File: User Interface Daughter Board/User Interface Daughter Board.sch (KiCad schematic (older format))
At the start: 27 parts, among them J1 Mother Board Conn, J2 Jack-DC, SW1 SW_Push_DPDT_2-5_3-4_1-4, SW2 SW_Push_Dual_1-3_2-4, SW3 SW_Push_Dual_1-3_2-4, SW4 SW_Push_Dual_1-3_2-4

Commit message: Update JST connectors
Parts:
- J1: footprint Naquadah_Generator:Daughter_Board_Vert_6_Pin_JST_Conn -> Connector_JST:JST_SH_BM06B-SRSS-TB_1x06-1MP_P1.00mm_Vertical
- WA1: footprint Naquadah_Generator:Wire_Assembly_Four -> Mechanical_LE:Wire_Assembly; symbol Naquadah_Generator:WireAssembly -> Mechanical_LE:WireAssembly; Manufacturer Part No. A06SR06SR30K305B -> A06SR06SR30K305A; Source Part No. 455-3019-ND -> 455-3007-ND
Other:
- note added: "6 pin at 1 mm spacing cable assembly.\nThe cable is reversed.\nThe mother board and daughter board\nuse the same foot prints."
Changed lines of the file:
@@
 F 0 "J1" H 4150 4150 50  0000 C CNN
 F 1 "Mother Board Conn" V 4600 4500 50  0000 C CNN
-F 2 "Naquadah_Generator:Daughter_Board_Vert_6_Pin_JST_Conn" H 4200 3850 50  0001 C CNN
+F 2 "Connector_JST:JST_SH_BM06B-SRSS-TB_1x06-1MP_P1.00mm_Vertical" H 4200 3850 50  0001 C CNN
 F 3 "http://www.jst-mfg.com/product/pdf/eng/eSH.pdf" H 4150 4550 50  0001 C CNN
 F 4 "Digikey" H 4150 4500 50  0001 C CNN "Source"
@@
 Ready Indicator
 $Comp
-L Naquadah_Generator:WireAssembly WA1
+L Mechanical_LE:WireAssembly WA1
 U 1 1 5EDA8160
-P 4900 6900
-F 0 "WA1" H 5278 6946 50  0000 L CNN
-F 1 "WireAssembly" H 5278 6855 50  0000 L CNN
-F 2 "Naquadah_Generator:Wire_Assembly_Four" H 4900 7000 50  0001 C CNN
-F 3 "http://www.jst-mfg.com/product/pdf/eng/eSR.pdf" H 4900 7000 50  0001 C CNN
-F 4 "6 Position Cable Assembly Rectangular Socket to Socket, Reversed 1.00' (304.80mm)" H 4900 6900 50  0001 C CNN "Description"
-F 5 "Digikey" H 4900 6900 50  0001 C CNN "Source"
-F 6 "455-3019-ND" H 4900 6900 50  0001 C CNN "Source Part No."
-F 7 "JST Sales America Inc." H 4900 6900 50  0001 C CNN "Manufacturer Name"
-F 8 "A06SR06SR30K305B" H 4900 6900 50  0001 C CNN "Manufacturer Part No."
-	1    4900 6900
+P 4950 6800
+F 0 "WA1" H 5328 6846 50  0000 L CNN
+F 1 "WireAssembly" H 5328 6755 50  0000 L CNN
+F 2 "Mechanical_LE:Wire_Assembly" H 4950 6900 50  0001 C CNN
+F 3 "https://gam-gec.com/wp-content/uploads/2018/10/GAM-012.pdf" H 4950 6900 50  0001 C CNN
+F 4 "6 Position Cable Assembly Rectangular Socket to Socket, Reversed 1.00' (304.80mm)" H 4950 6800 50  0001 C CNN "Description"
+F 5 "Digikey" H 4950 6800 50  0001 C CNN "Source"
+F 6 "455-3007-ND" H 4950 6800 50  0001 C CNN "Source Part No."
+F 7 "JST Sales America Inc." H 4950 6800 50  0001 C CNN "Manufacturer Name"
+F 8 "A06SR06SR30K305A" H 4950 6800 50  0001 C CNN "Manufacturer Part No."
+	1    4950 6800
 	1    0    0    -1
 $EndComp
@@
 	8150 1900 8050 1900
 Connection ~ 8150 1900
+Text Notes 4650 7250 0    50   ~ 0
+6 pin at 1 mm spacing cable assembly.\nThe cable is reversed.\nThe mother board and daughter board\nuse the same foot prints.
 $EndSCHEMATC

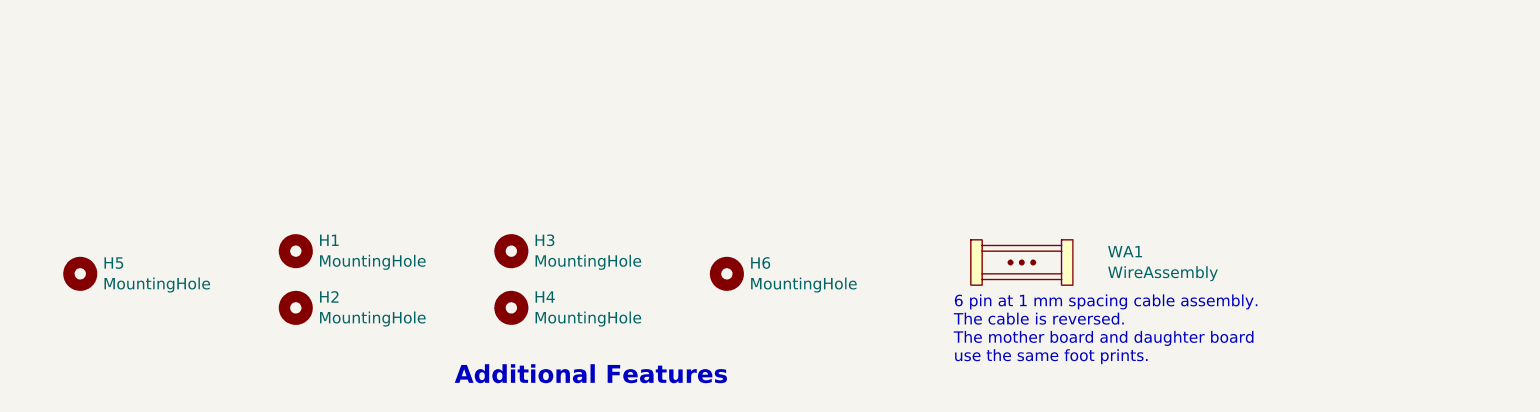
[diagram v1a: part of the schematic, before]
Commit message: Updated fiducials.
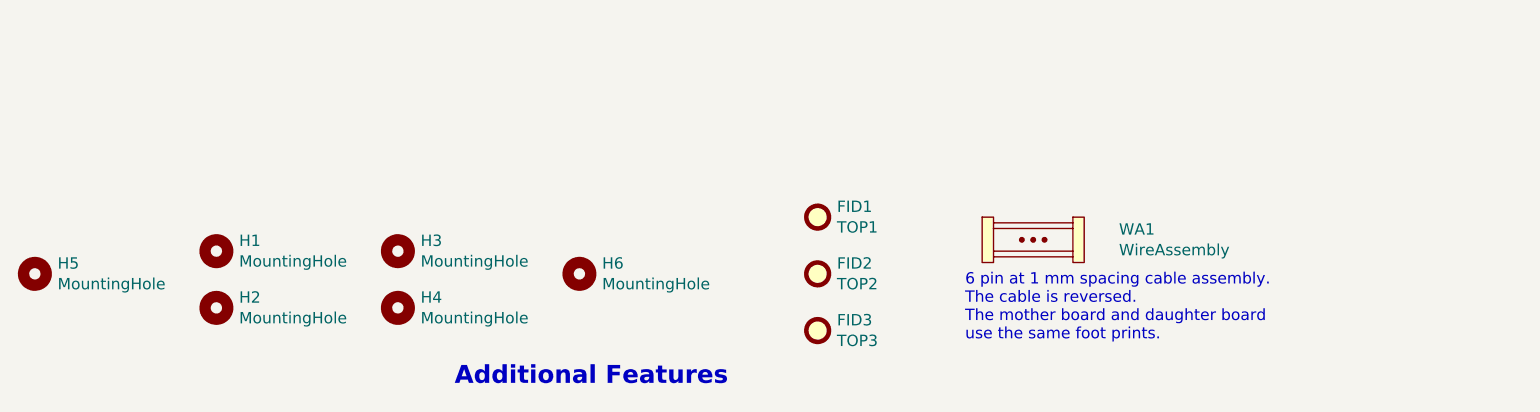
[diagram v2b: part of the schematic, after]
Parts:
- added FID1, FID2, FID3: Fiducial, Fiducial_LE:Fiducial_1mm_Mask2mm, symbol Mechanical_LE:Fiducial
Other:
- moved on the sheet: H1, H2, H3, H4, H5, H6, WA1
